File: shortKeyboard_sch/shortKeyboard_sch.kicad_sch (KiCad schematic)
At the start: 19 parts, among them J1 MPU5060 2.54 1x8, J10 In, J11 Conn_01x06, J12 Out, J2 TP4056 bat/out 2.54, J3 TP4056 in 2.54 1x6, J4 USB Power Data 2.54, J5 esp32 left 2.54 MALE, J6 esp32 right 2.54 MALE, J7 ESP32 USB 2.54 Data, J8 Li-Ion Batter 2.54, J9 Buttons Connector 2.54

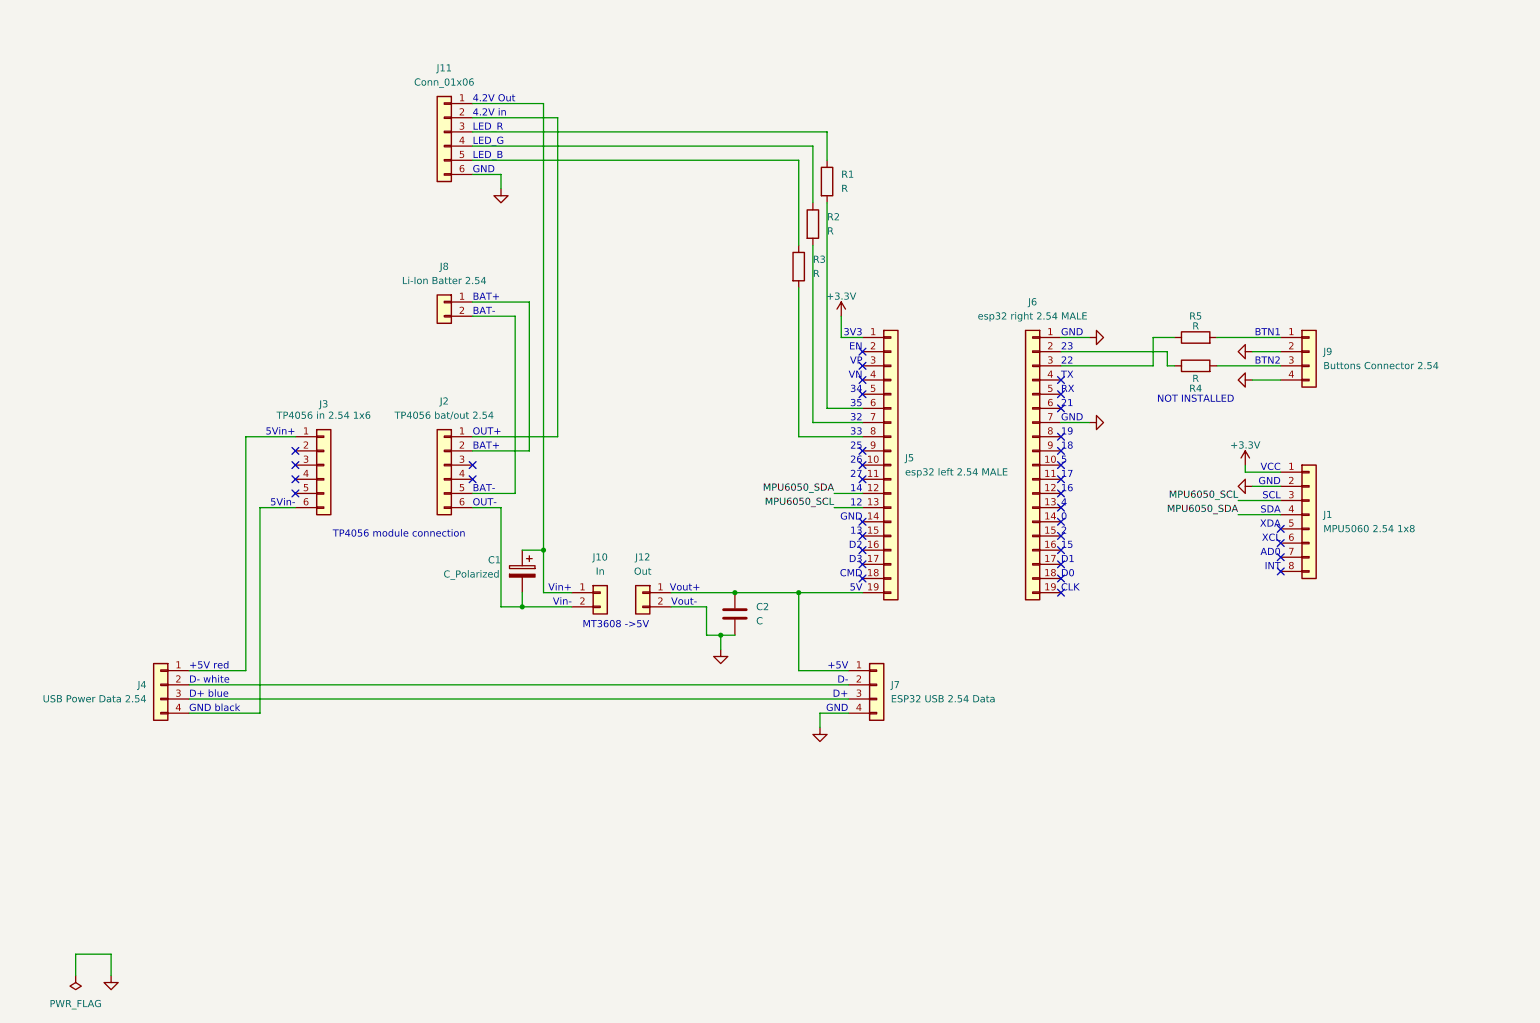
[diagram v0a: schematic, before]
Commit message: intermediate new pcb version again
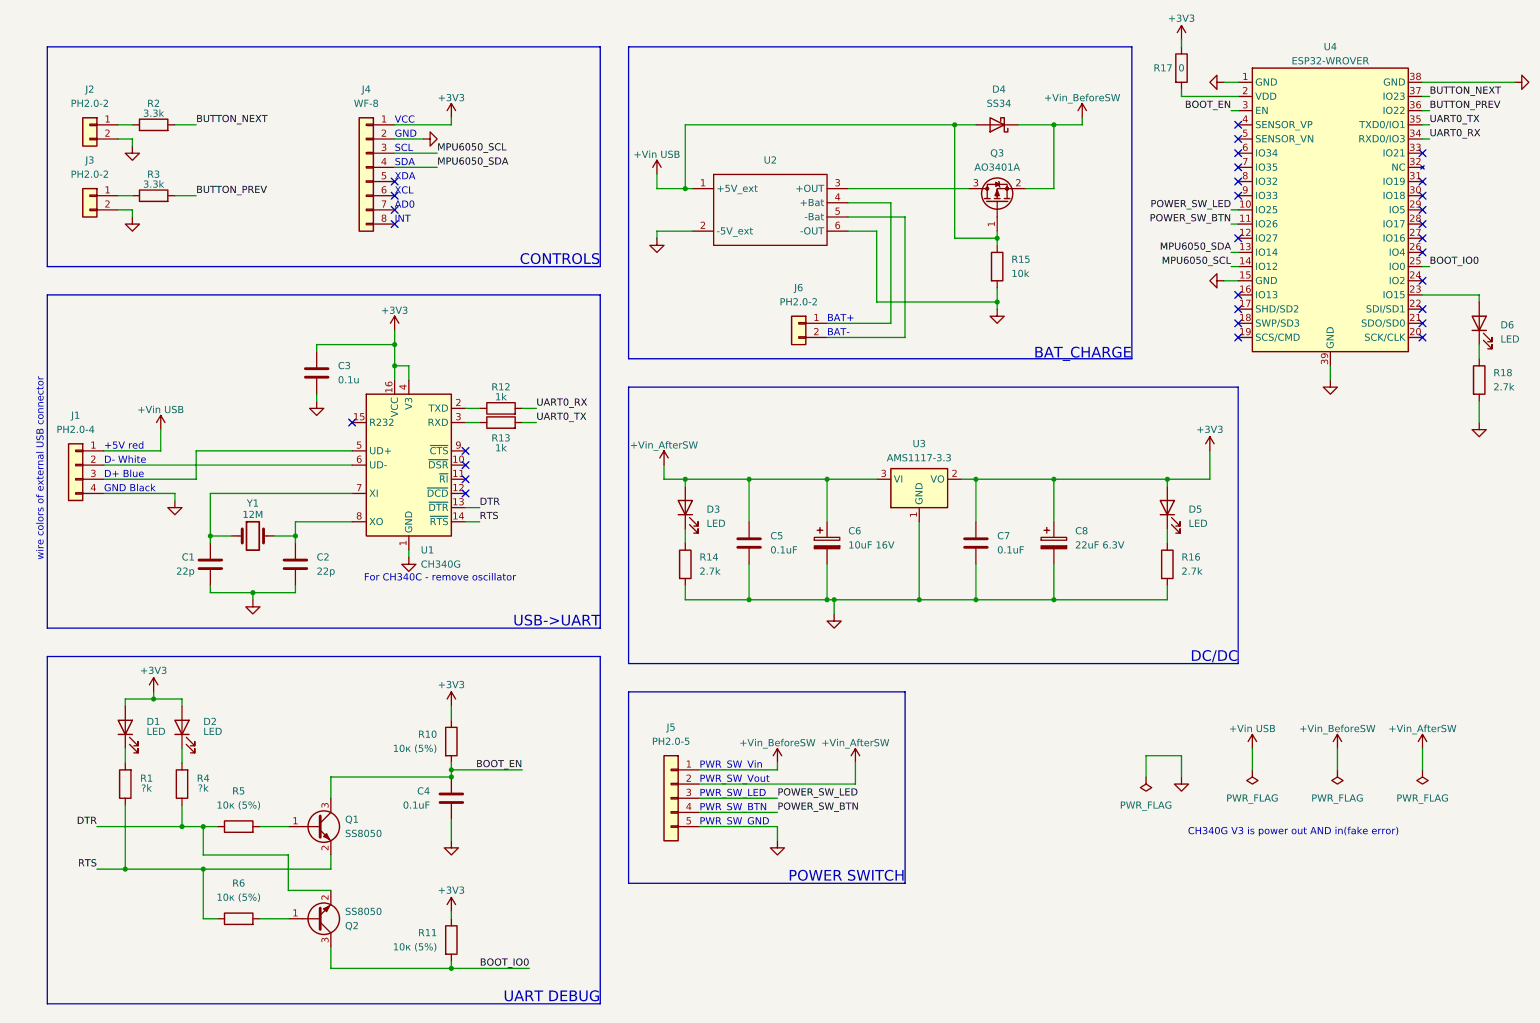
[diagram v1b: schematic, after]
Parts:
- removed C1: C_Polarized, symbol Device:C_Polarized
- removed J1: MPU5060 2.54 1x8, symbol Connector_Generic:Conn_01x08
- removed J10: In, symbol Connector_Generic:Conn_01x02
- removed J11: Conn_01x06, symbol Connector_Generic:Conn_01x06
- removed J12: Out, symbol Connector_Generic:Conn_01x02
- removed J2: TP4056 bat/out 2.54, symbol Connector_Generic:Conn_01x06
- removed J3: TP4056 in 2.54 1x6, symbol Connector_Generic:Conn_01x06
- removed J4: USB Power Data 2.54, symbol Connector_Generic:Conn_01x04
- removed J5: esp32 left 2.54 MALE, symbol Connector_Generic:Conn_01x19
- removed J6: esp32 right 2.54 MALE, symbol Connector_Generic:Conn_01x19
- removed J7: ESP32 USB 2.54 Data, symbol Connector_Generic:Conn_01x04
- removed J8: Li-Ion Batter 2.54, symbol Connector_Generic:Conn_01x02
- removed J9: Buttons Connector 2.54, symbol Connector_Generic:Conn_01x04
- added C1: 22p, Capacitor_SMD:C_0805_2012Metric_Pad1.18x1.45mm_HandSolder, symbol Device:C
- added C3: 0.1u, Capacitor_SMD:C_0805_2012Metric_Pad1.18x1.45mm_HandSolder, symbol Device:C
- added C4, C5, C7: 0.1uF, Capacitor_SMD:C_0805_2012Metric_Pad1.18x1.45mm_HandSolder, symbol Device:C
- added C6: 10uF 16V, Capacitor_Tantalum_SMD:CP_EIA-3216-18_Kemet-A_HandSolder, symbol Device:C_Polarized
- added C8: 22uF 6.3V, Capacitor_Tantalum_SMD:CP_EIA-3216-18_Kemet-A_HandSolder, symbol Device:C_Polarized
- added D1, D2, D3, D5, D6: LED, LED_SMD:LED_0805_2012Metric_Pad1.15x1.40mm_HandSolder, symbol Device:LED
- added D4: SS34, Diode_SMD:D_SMA, symbol Diode:SS34
- added J1: PH2.0-4, lw_kicadLib:PH2.0-4, symbol lw_kicadLib:PH2.0-4
- added J2, J3, J6: PH2.0-2, lw_kicadLib:PH2.0-2, symbol lw_kicadLib:PH2.0-2
- added J4: WF-8, lw_kicadLib:WF-8, symbol lw_kicadLib:WF-8
- added J5: PH2.0-5, lw_kicadLib:PH2.0-5, symbol lw_kicadLib:PH2.0-5
- added Q1, Q2: SS8050, Package_TO_SOT_SMD:SOT-23, symbol Transistor_BJT:SS8050
- added Q3: AO3401A, Package_TO_SOT_SMD:SOT-23, symbol Transistor_FET:AO3401A
- added R10, R11, R6: 10к (5%), Resistor_SMD:R_0805_2012Metric_Pad1.20x1.40mm_HandSolder, symbol Device:R
- added R12, R13: 1k, Resistor_SMD:R_0805_2012Metric_Pad1.20x1.40mm_HandSolder, symbol Device:R
- added R14, R16, R18: 2.7k, Resistor_SMD:R_0805_2012Metric_Pad1.20x1.40mm_HandSolder, symbol Device:R
- added R15: 10k, Resistor_SMD:R_0805_2012Metric_Pad1.20x1.40mm_HandSolder, symbol Device:R
- added R17: 0, Resistor_SMD:R_0805_2012Metric_Pad1.20x1.40mm_HandSolder, symbol Device:R
- added U1: CH340G, Package_SO:SOIC-16_3.9x9.9mm_P1.27mm, symbol Interface_USB:CH340G
- added U2: (no value), lw_kicadLib:TP4056_Module_CD_MicroUsb, symbol lw_kicadLib:TP4056_Module
- added U3: AMS1117-3.3, Package_TO_SOT_SMD:SOT-223-3_TabPin2, symbol Regulator_Linear:AMS1117-3.3
- added U4: ESP32-WROVER, lw_kicadLib:ESP32-WROVER-handSoldering, symbol lw_kicadLib:ESP32-WROVER
- added Y1: 12M, Crystal:Crystal_SMD_HC49-SD_HandSoldering, symbol Device:Crystal
- C2: value C -> 22p; footprint (none) -> Capacitor_SMD:C_0805_2012Metric_Pad1.18x1.45mm_HandSolder
- R1, R4: value R -> ?k; footprint (none) -> Resistor_SMD:R_0805_2012Metric_Pad1.20x1.40mm_HandSolder
- R2, R3: value R -> 3.3k; footprint (none) -> Resistor_SMD:R_0805_2012Metric_Pad1.20x1.40mm_HandSolder
- R5: value R -> 10к (5%); footprint (none) -> Resistor_SMD:R_0805_2012Metric_Pad1.20x1.40mm_HandSolder
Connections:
- net GND: now also C1.2, C3.2, C4.2, C5.2, C6.2, C7.2, C8.2, J1.4 (Pin_1), J2.2 (Pin_2), J3.2 (Pin_2), J4.2 (Pin_2), J5.5 (Pin_1), R14.2, R15.2, R16.2, R18.2, U1.1 (GND), U2.2 (-5V_ext), U2.6 (-OUT), U3.1 (GND), U4.1 (GND), U4.15 (GND), U4.38 (GND), U4.39 (GND)
- net MPU6050_SCL: now also J4.3 (Pin_3), U4.14 (IO12)
- net MPU6050_SDA: now also J4.4 (Pin_4), U4.13 (IO14)
- net DTR: now reaches R4.1
- net DTR: now also R5.1, Q2.2 (E), U1.13 (~{DTR})
- net at R4.2: now also D2.1 (K)
- net at R5.2: now also Q1.1 (B)
- net RTS: now reaches R1.1
- net RTS: now also Q1.2 (E), R6.1, U1.14 (~{RTS})
- net at R2.1: now also J2.1 (Pin_1)
- net at R3.1: now also J3.1 (Pin_1)
- net at C2.1: now also U1.8 (XO), Y1.2
- net at R1.2: now also D1.1 (K)
- net BUTTON_PREV: now reaches R3.2
- net BUTTON_PREV: now also U4.36 (IO22)
- net BUTTON_NEXT: now reaches R2.2
- net BUTTON_NEXT: now also U4.37 (IO23)
- new net: R12.1, U1.2 (TXD)
- new net: R13.1, U1.3 (RXD)
- new net: J1.3 (Pin_2), U1.5 (UD+)
- new net: J1.2 (Pin_1), U1.6 (UD-)
- new net: C1.1, U1.7 (XI), Y1.1
- new net: D3.1 (K), R14.1
- new net: D5.1 (K), R16.1
- new net: Q2.1 (B), R6.2
- new net: Q3.3 (D), U2.3 (+OUT)
- new net: J6.1 (Pin_1), U2.4 (+Bat)
- new net: J6.2 (Pin_2), U2.5 (-Bat)
- new net: R17.2, U4.2 (VDD)
- new net: D6.1 (K), R18.1
- new net: D6.2 (A), U4.23 (IO15)
- new net +3V3: C3.1, C7.1, C8.1, D1.2 (A), D2.2 (A), D5.2 (A), J4.1 (Pin_1), R10.1, R11.1, R17.1, U1.16 (VCC), U1.4 (V3), U3.2 (VO)
- new net +Vin USB: D4.2 (A), J1.1 (Pin_1), Q3.1 (G), R15.1, U2.1 (+5V_ext)
- new net +Vin_AfterSW: C5.1, C6.1, D3.2 (A), J5.2 (Pin_1), U3.3 (VI)
- new net +Vin_BeforeSW: D4.1 (K), J5.1 (Pin_1), Q3.2 (S)
- new net BOOT_EN: C4.1, Q1.3 (C), R10.2, U4.3 (EN)
- new net BOOT_IO0: Q2.3 (C), R11.2, U4.25 (IO0)
- new net POWER_SW_BTN: J5.4 (Pin_1), U4.11 (IO26)
- new net POWER_SW_LED: J5.3 (Pin_2), U4.10 (IO25)
- new net UART0_RX: R12.2, U4.34 (RXD0/IO3)
- new net UART0_TX: R13.2, U4.35 (TXD0/IO1)
- no-connect marks 37 -> 31
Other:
- note added: "BAT_CHARGE"
- note added: "CH340G V3 is power out AND in(fake error)"
- note added: "CONTROLS"
- note added: "D+ Blue"
- note added: "D- White"
- note added: "DC/DC"
- note added: "For CH340C - remove oscillator"
- note added: "GND Black"
- note added: "POWER SWITCH"
- note added: "PWR_SW_BTN"
- note added: "PWR_SW_GND"
- note added: "PWR_SW_LED"
- note added: "PWR_SW_Vin"
- note added: "PWR_SW_Vout"
- note added: "UART DEBUG"
- note added: "USB->UART"
- note added: "wire colors of external USB connector"
- note removed: "+5V"
- note removed: "0"
- note removed: "12"
- note removed: "13"
- note removed: "14"
- note removed: "15"
- note removed: "16"
- note removed: "17"
- note removed: "18"
- note removed: "19"
- note removed: "2"
- note removed: "21"
- note removed: "22"
- note removed: "23"
- note removed: "25"
- note removed: "26"
- note removed: "27"
- note removed: "32"
- note removed: "33"
- note removed: "34"
- note removed: "35"
- note removed: "3V3"
- note removed: "4"
- note removed: "4.2V Out"
- note removed: "4.2V in"
- note removed: "5"
- note removed: "5V"
- note removed: "5Vin+"
- note removed: "5Vin-"
- note removed: "BTN1"
- note removed: "BTN2"
- note removed: "CLK"
- note removed: "CMD"
- note removed: "D+"
- note removed: "D+ blue"
- note removed: "D-"
- note removed: "D- white"
- note removed: "D0"
- note removed: "D1"
- note removed: "D2"
- note removed: "D3"
- note removed: "EN"
- note removed: "GND black"
- note removed: "LED_B"
- note removed: "LED_G"
- note removed: "LED_R"
- note removed: "MT3608 ->5V"
- note removed: "NOT INSTALLED"
- note removed: "OUT+"
- note removed: "OUT-"
- note removed: "RX"
- note removed: "TP4056 module connection"
- note removed: "TX"
- note removed: "VN"
- note removed: "VP"
- note removed: "Vin+"
- note removed: "Vin-"
- note removed: "Vout+"
- note removed: "Vout-"
